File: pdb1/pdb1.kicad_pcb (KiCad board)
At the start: 2 copper layers, 99.1 x 17.8 mm, 24 parts, among them P1 CONN_XT60, P2 CONN_XT60, P3 CONN_02X03, P4 CONN_01X02, P5 CONN_01X02, Q2 BUK9Y4R8-60E, U1 INA169, U2 NSI45020AT1G, U3 NSI45020AT1G, U4 LM3480-3.3, U5 74LVC1G08, U7 MIC5014, U8 NSI45020AT1G

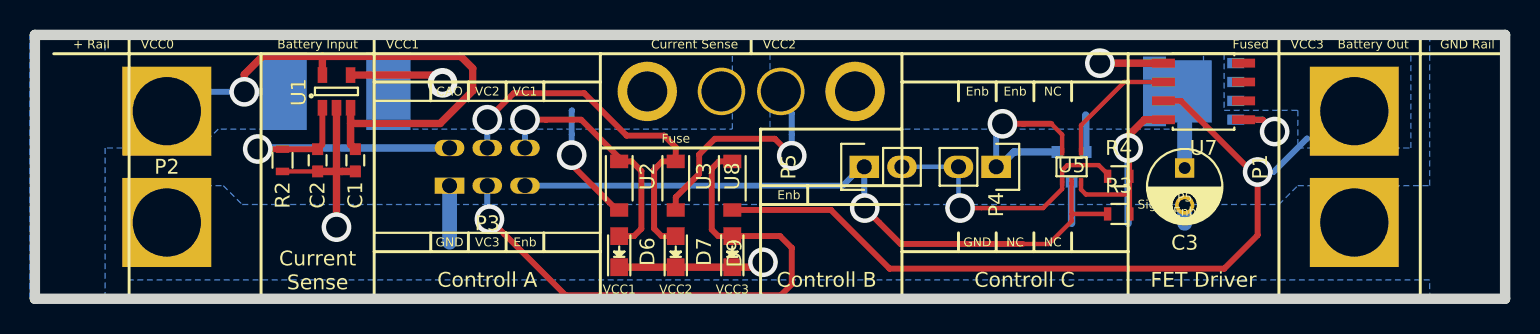
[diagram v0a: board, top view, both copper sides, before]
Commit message: test
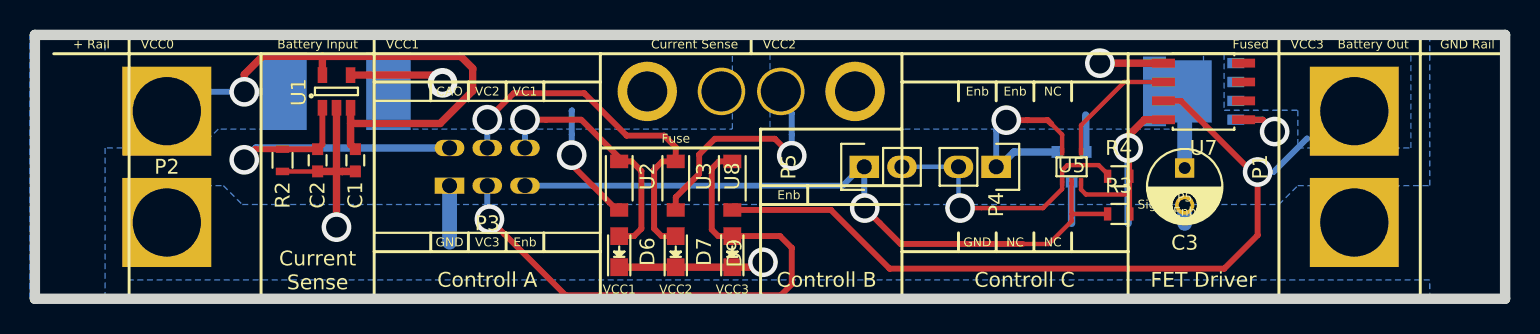
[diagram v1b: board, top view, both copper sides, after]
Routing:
- net /channel/current_sensor/sense: track 19.9 -> 22.3 mm
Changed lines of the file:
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@@
-(kicad_pcb (version 4) (host pcbnew 4.0.4-stable)
+(kicad_pcb (version 4) (host pcbnew 4.0.4+e1-6308~48~ubuntu16.04.1-stable)
   (general
     (links 54)
     (no_connects 0)
-    (area 50.449999 50.449999 150.210001 68.930001)
+    (area 50.449999 46.015 150.210001 68.930001)
     (thickness 1.6)
     (drawings 75)
-    (tracks 186)
+    (tracks 187)
     (zones 0)
     (modules 24)
@@
   )
   (setup
-    (last_trace_width 0.5)
+    (last_trace_width 0.25)
     (user_trace_width 0.3)
     (user_trace_width 0.4)
@@
   (segment (start 71.508586 60.0075) (end 71.12 60.0075) (width 0.5) (layer F.Cu) (net 2))
   (via (at 71.12 63.754) (size 2) (drill 1.4) (layers F.Cu B.Cu) (net 2))
-  (segment (start 78.74 58.42) (end 65.883551 58.42) (width 0.5) (layer B.Cu) (net 3))
-  (segment (start 65.883551 58.42) (end 65.815282 58.488269) (width 0.5) (layer B.Cu) (net 3))
-  (segment (start 67.484392 58.501086) (end 65.828099 58.501086) (width 0.4) (layer F.Cu) (net 3))
-  (segment (start 65.828099 58.501086) (end 65.815282 58.488269) (width 0.4) (layer F.Cu) (net 3))
-  (via (at 65.815282 58.488269) (size 2) (drill 1.4) (layers F.Cu B.Cu) (net 3))
+  (segment (start 65.624384 58.501086) (end 64.908756 59.216714) (width 0.4) (layer F.Cu) (net 3))
+  (segment (start 67.484392 58.501086) (end 65.624384 58.501086) (width 0.4) (layer F.Cu) (net 3))
+  (segment (start 65.70547 58.42) (end 64.908756 59.216714) (width 0.5) (layer B.Cu) (net 3))
+  (segment (start 78.74 58.42) (end 65.70547 58.42) (width 0.5) (layer B.Cu) (net 3))
+  (via (at 64.908756 59.216714) (size 2) (drill 1.4) (layers F.Cu B.Cu) (net 3))
   (segment (start 70.17 55.71) (end 70.17 58.181086) (width 0.4) (layer F.Cu) (net 3))
   (segment (start 70.17 58.181086) (end 69.85 58.501086) (width 0.4) (layer F.Cu) (net 3))
@@
   (via (at 113.137105 62.470628) (size 2) (drill 1.4) (layers F.Cu B.Cu) (net 12))
   (segment (start 109.22 59.69) (end 113.03 59.69) (width 0.3) (layer B.Cu) (net 12))
+  (segment (start 115.57 57.226029) (end 116.251041 56.544988) (width 0.4) (layer B.Cu) (net 13))
+  (segment (start 115.57 59.69) (end 115.57 57.226029) (width 0.4) (layer B.Cu) (net 13))
+  (segment (start 119.036735 56.544988) (end 117.665254 56.544988) (width 0.4) (layer F.Cu) (net 13))
+  (segment (start 119.283859 56.792112) (end 119.036735 56.544988) (width 0.4) (layer F.Cu) (net 13))
+  (segment (start 117.665254 56.544988) (end 116.251041 56.544988) (width 0.4) (layer F.Cu) (net 13))
+  (via (at 116.251041 56.544988) (size 2) (drill 1.4) (layers F.Cu B.Cu) (net 13))
   (segment (start 120.015 58.674) (end 120.015 57.523253) (width 0.3) (layer F.Cu) (net 13))
   (segment (start 120.015 57.523253) (end 119.283859 56.792112) (width 0.3) (layer F.Cu) (net 13))
-  (segment (start 119.283859 56.792112) (end 117.408322 56.792112) (width 0.4) (layer F.Cu) (net 13))
-  (segment (start 117.408322 56.792112) (end 115.994109 56.792112) (width 0.4) (layer F.Cu) (net 13))
-  (segment (start 115.57 57.216221) (end 115.994109 56.792112) (width 0.4) (layer B.Cu) (net 13))
-  (segment (start 115.57 59.69) (end 115.57 57.216221) (width 0.4) (layer B.Cu) (net 13))
-  (via (at 115.994109 56.792112) (size 2) (drill 1.4) (layers F.Cu B.Cu) (net 13))
   (segment (start 119.7 58.68924) (end 116.765659 58.68924) (width 0.5) (layer B.Cu) (net 13))
   (segment (start 116.765659 58.68924) (end 115.764899 59.69) (width 0.5) (layer B.Cu) (net 13))
